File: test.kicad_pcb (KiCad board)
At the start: 2 copper layers, 40.6 x 53 mm, 30 parts, among them P1 CONN5, P10 CONN_01X05, P2 USB_Micro, P3 CONN_VCC, P4 CONN_01X03, P5 CONN_01X03, P6 CONN_01X01, P7 CONN_01X01, P8 CONN_01X01, P9 CONN_01X02, U1 TPS61800 module, U2 G5177 module, U3 TMP432, U4 LDO_3V5, U5 TP5000 Charger

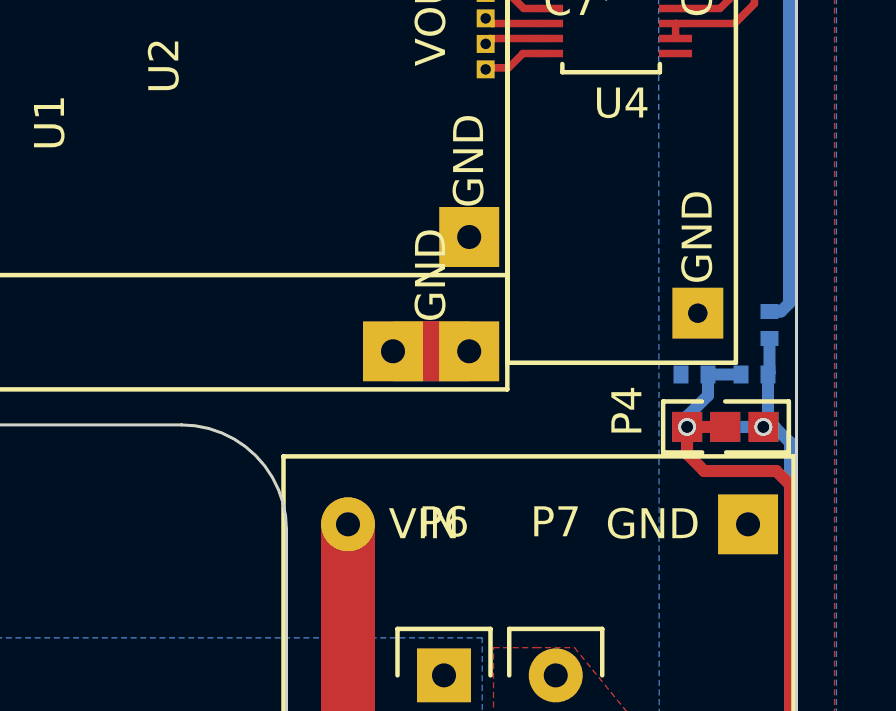
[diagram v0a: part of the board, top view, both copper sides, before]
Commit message: PCB in v6
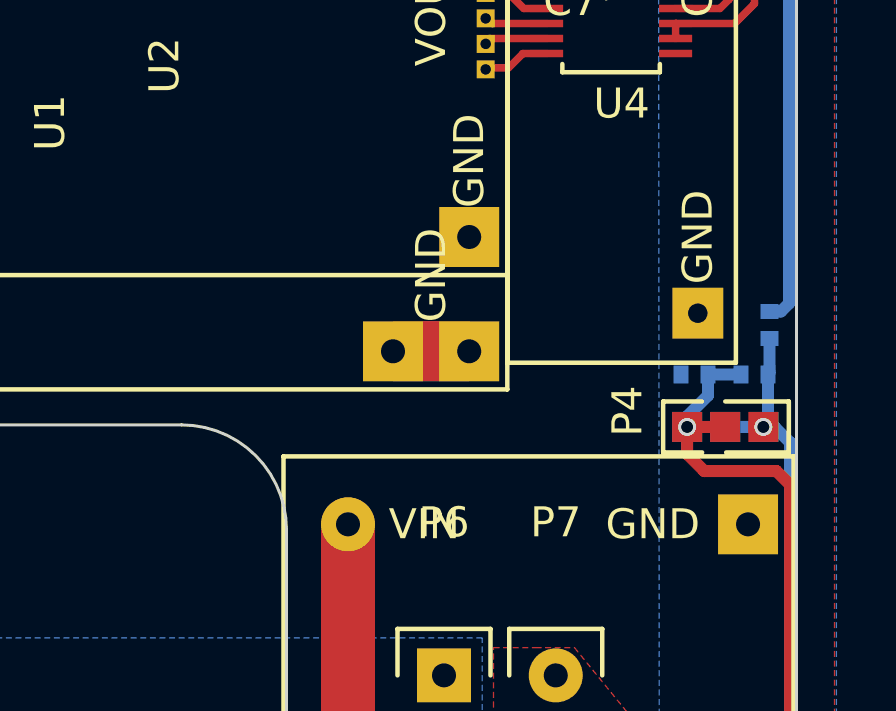
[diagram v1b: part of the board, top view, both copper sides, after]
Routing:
- net (no net): track 3.13 -> 0.00 mm
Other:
- net class Default removed
